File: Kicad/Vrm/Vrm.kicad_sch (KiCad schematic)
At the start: 7 parts, among them J1 Screw_Terminal_01x04, J2 Screw_Terminal_01x04, J3 Screw_Terminal_01x02, Q1 ZVN4106F

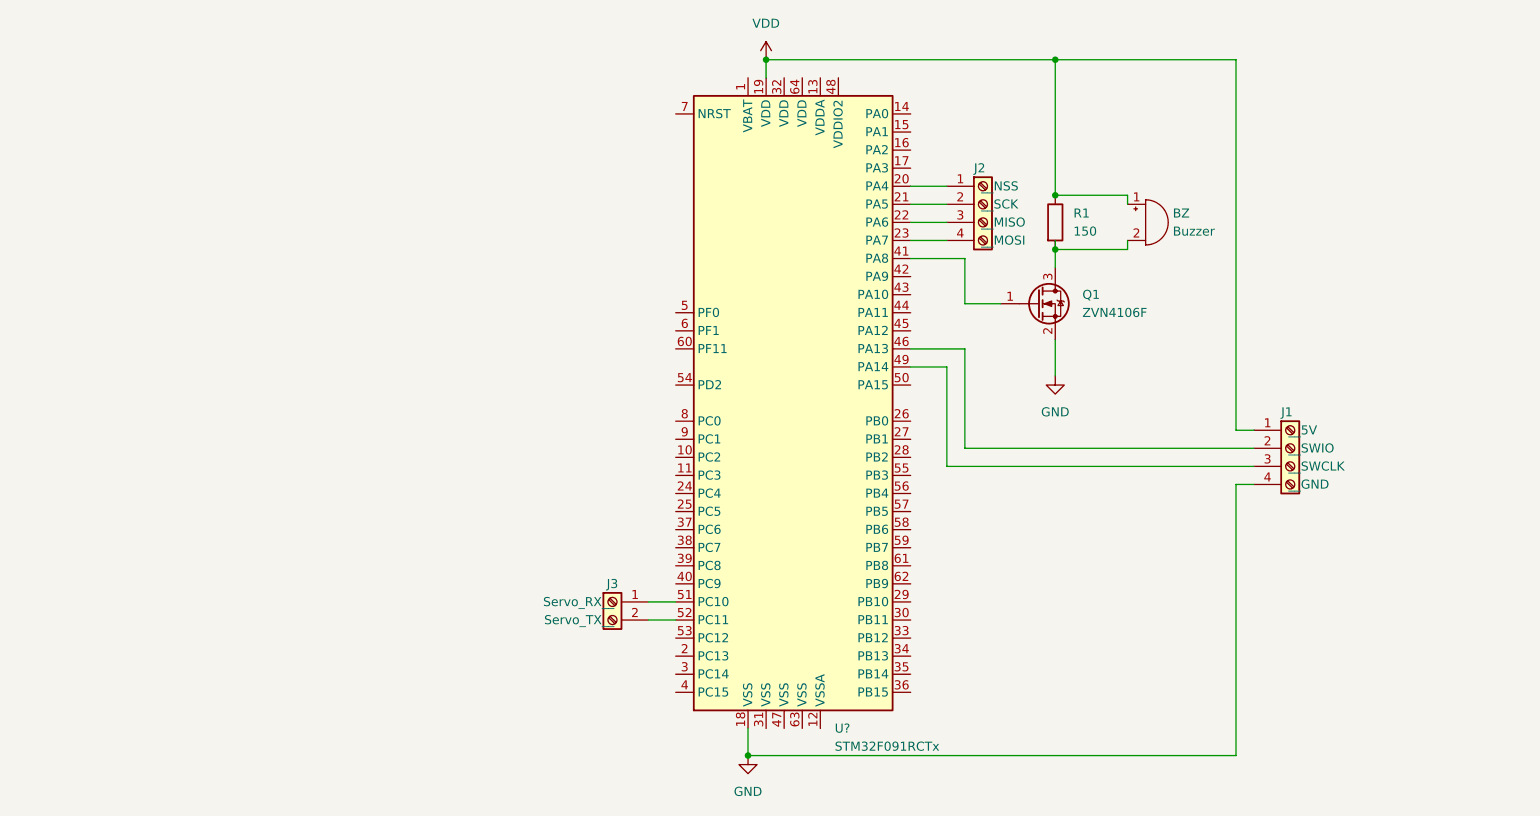
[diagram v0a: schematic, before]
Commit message: Updated Schematic
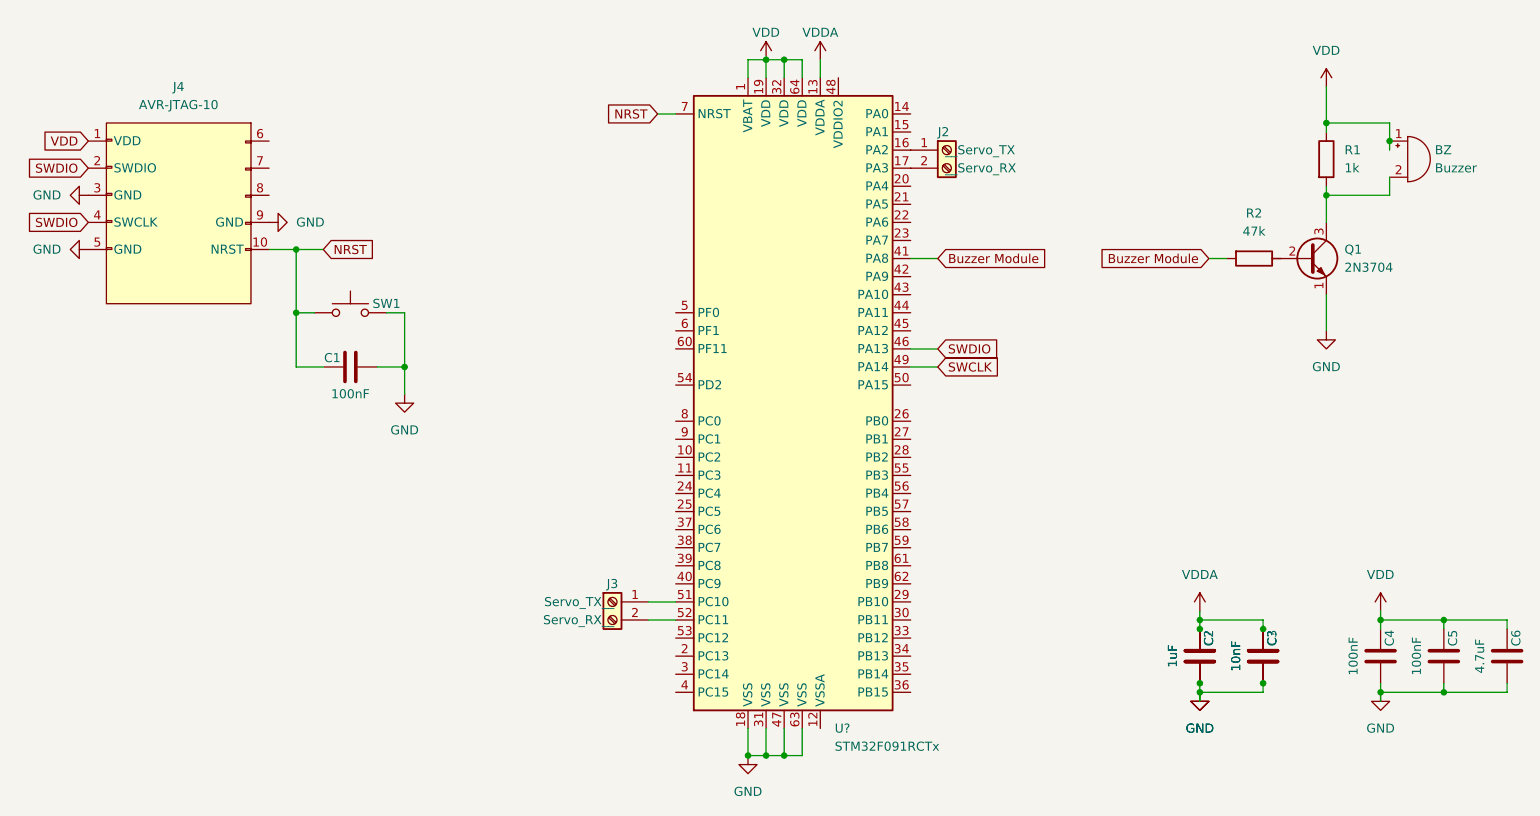
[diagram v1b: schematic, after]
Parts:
- removed J1, J2: Screw_Terminal_01x04, symbol Connector:Screw_Terminal_01x04
- removed Q1: ZVN4106F, Package_TO_SOT_SMD:SOT-23, symbol Transistor_FET:ZVN4106F
- added C1, C4, C5: 100nF, symbol Device:C
- added C2, C?: 1uF, symbol Device:C
- added C3, C?: 10nF, symbol Device:C
- added C6: 4.7uF, symbol Device:C
- added J2: Screw_Terminal_01x02, symbol Connector:Screw_Terminal_01x02
- added J4: AVR-JTAG-10, symbol Connector:AVR-JTAG-10
- added Q1: 2N3704, Package_TO_SOT_THT:TO-92_Inline, symbol Transistor_BJT:2N3904
- added R2: 47k, symbol Device:R
- added SW1: Switch, symbol Switch:SW_Push
- R1: value 150 -> 1k
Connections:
- net GND: now also U?.31 (VSS), U?.47 (VSS), U?.63 (VSS), C1.2, C2.2, C3.2, C4.2, C5.2, C6.2, C?.2, C?.2, J4.3 (GND), J4.5 (GND), J4.9 (GND), Q1.1 (E), SW1.2
- net VDD: now also U?.1 (VBAT), U?.32 (VDD), U?.64 (VDD), C4.1, C5.1, C6.1, J4.1 (VDD)
- net Buzzer Module: now reaches U?.41 (PA8)
- net Buzzer Module: now also R2.2
- net at BZ.2 (+), R1.2: now also Q1.3 (C)
- net VDDA: now reaches U?.13 (VDDA)
- net VDDA: now also C2.1, C3.1, C?.1, C?.1
- net at U?.16 (PA2): now also J2.1 (__Servo_TX)
- net at U?.17 (PA3): now also J2.2 (__Servo_RX)
- net SWDIO: now reaches U?.46 (PA13)
- net SWDIO: now also J4.2 (SWDIO), J4.4 (SWCLK)
- net SWCLK: now reaches U?.49 (PA14)
- net NRST: now reaches U?.7 (NRST)
- net NRST: now also C1.1, J4.10 (NRST), SW1.1
